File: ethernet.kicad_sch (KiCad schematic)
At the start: 6 parts, among them J1 ARJM11C7-502-AB-ER2-T

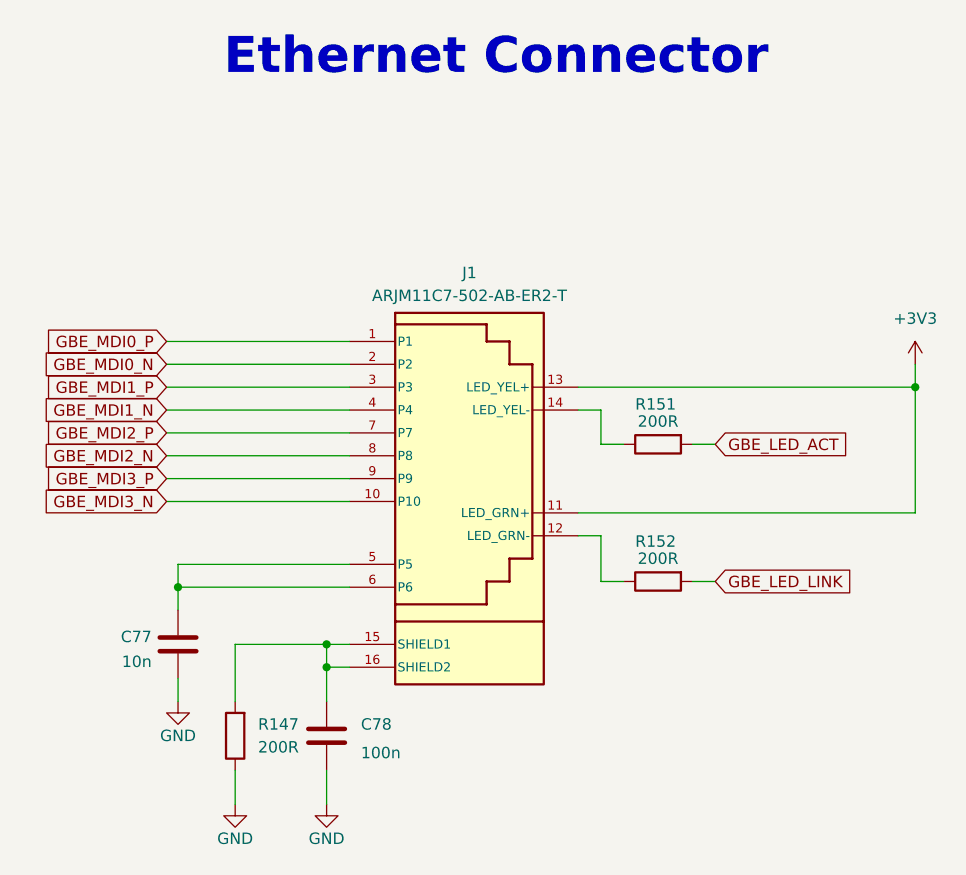
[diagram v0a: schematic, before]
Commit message: Schematic Done
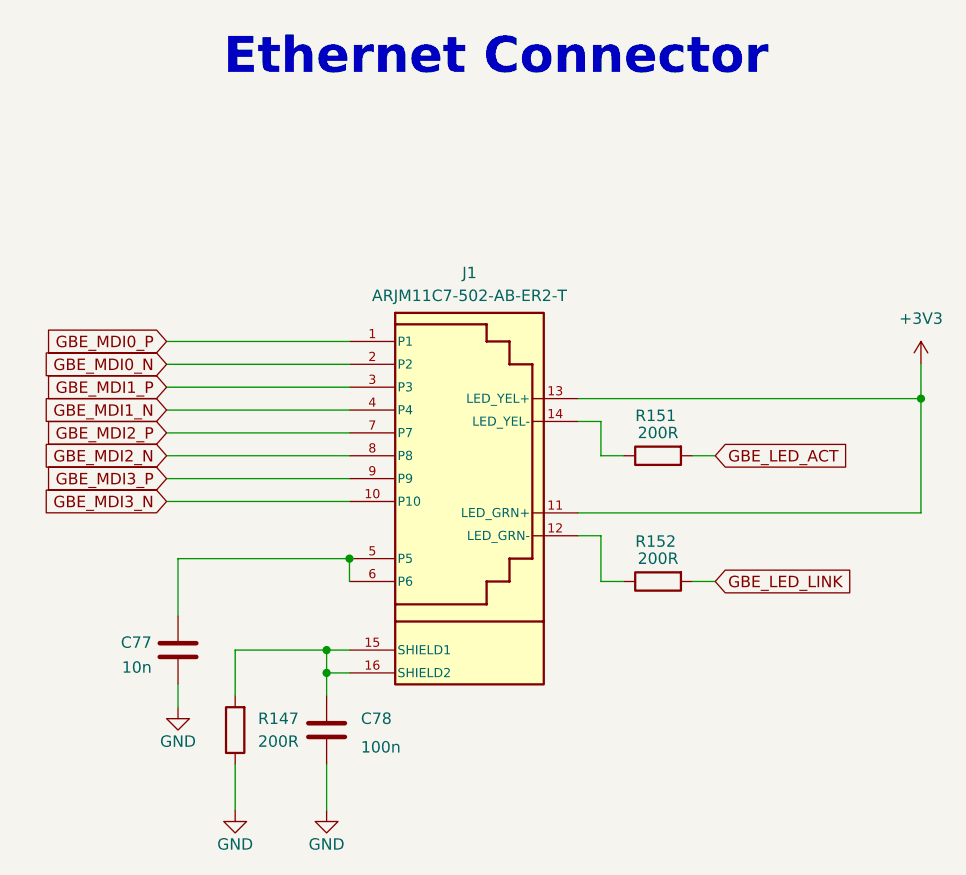
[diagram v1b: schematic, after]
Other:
- moved on the sheet: C77, C78, R147, R151
